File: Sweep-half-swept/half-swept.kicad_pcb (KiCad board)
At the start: 2 copper layers, 108.6 x 86.9 mm, 26 parts, among them J2 AudioJack4dpb, SW10 SW_Push, SW11 SW_Push, SW12 SW_Push, SW14 SW_Push, SW15 SW_Push, SW16 SW_Push, SW17 SW_Push, SW18 SW_Push, SW2 SW_Push, SW2 SW_SPDT, SW20 SW_Push, SW21 SW_Push, SW3 SW_Push, SW4 SW_Push, SW5 SW_Push, SW6 SW_Push, SW8 SW_Push, SW9 SW_Push, U1 ProMicro-kbd

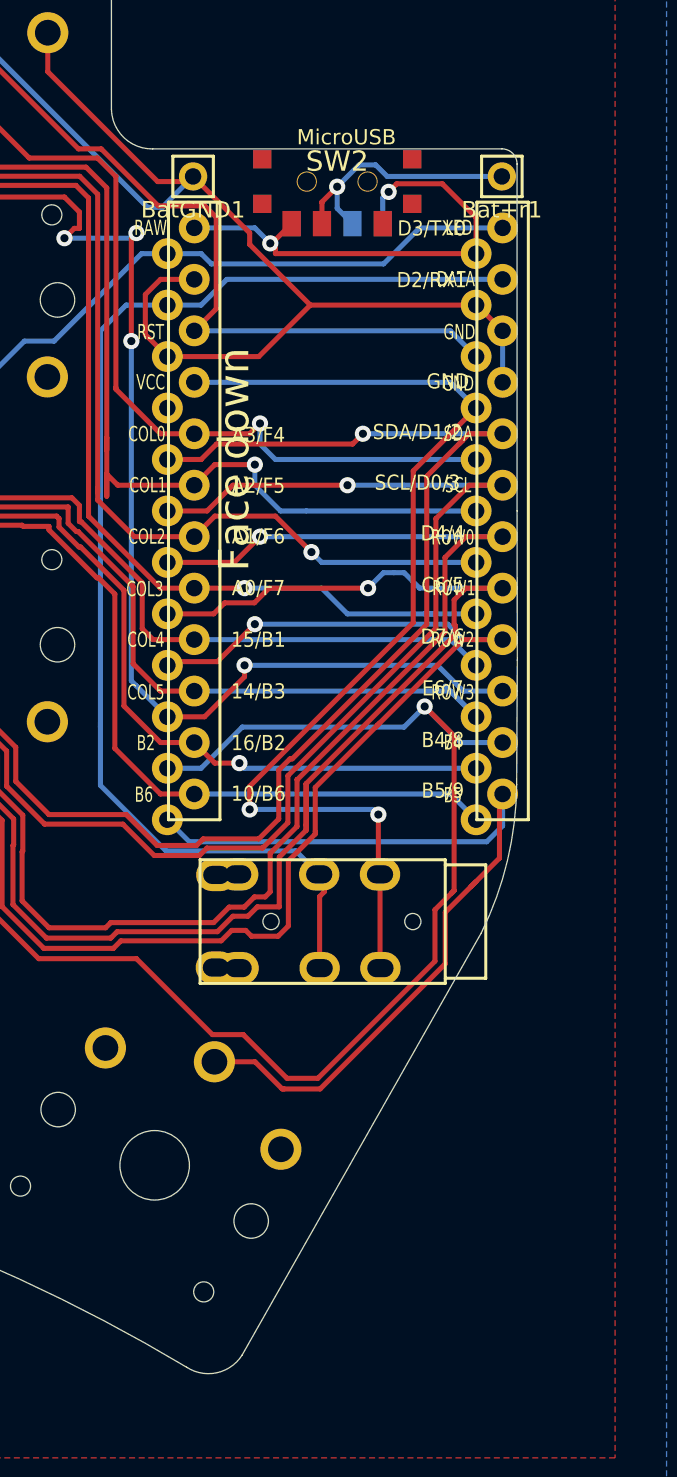
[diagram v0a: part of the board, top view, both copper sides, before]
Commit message: Update silk and edge cuts
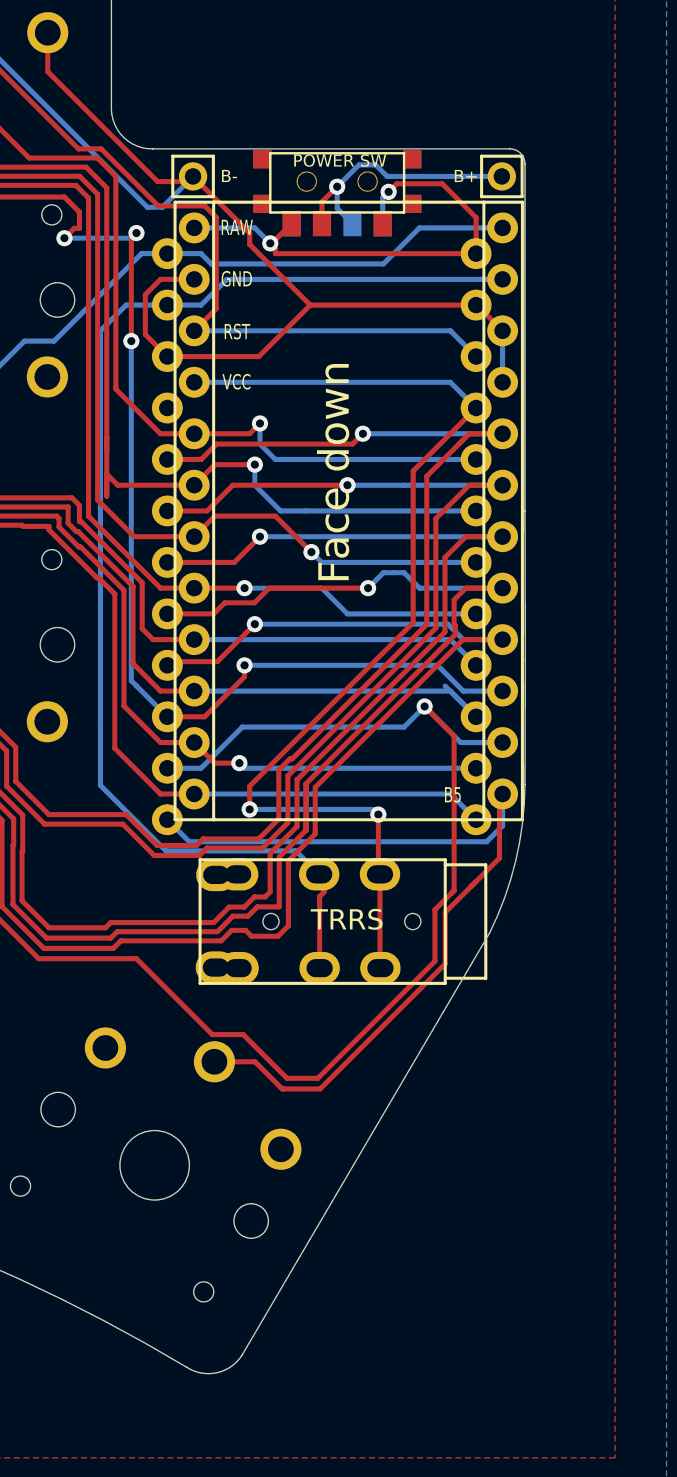
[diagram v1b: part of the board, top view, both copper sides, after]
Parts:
- POWER SW: renamed from SW_POWERR1
- renumbered Bat+r1 to B+, BatGND1 to B-
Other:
- board size 108.6 x 86.9 mm -> 109 x 86.9 mm
- board text added: "B+"
- board text added: "B-"
- board text added: "POWER SW"
- board text added: "TRRS"
